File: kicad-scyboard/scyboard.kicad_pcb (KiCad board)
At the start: 2 copper layers, 144 x 96.5 mm, 76 parts

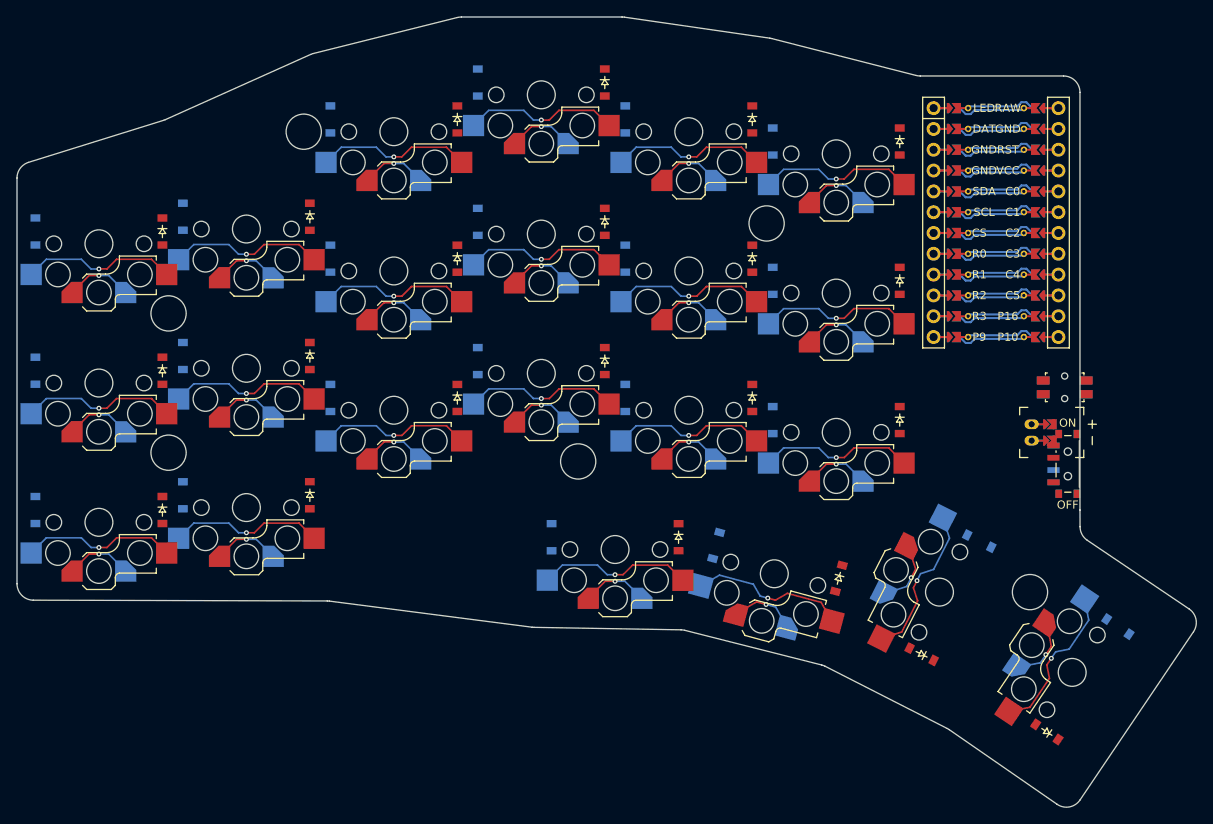
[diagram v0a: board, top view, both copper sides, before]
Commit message: Compile
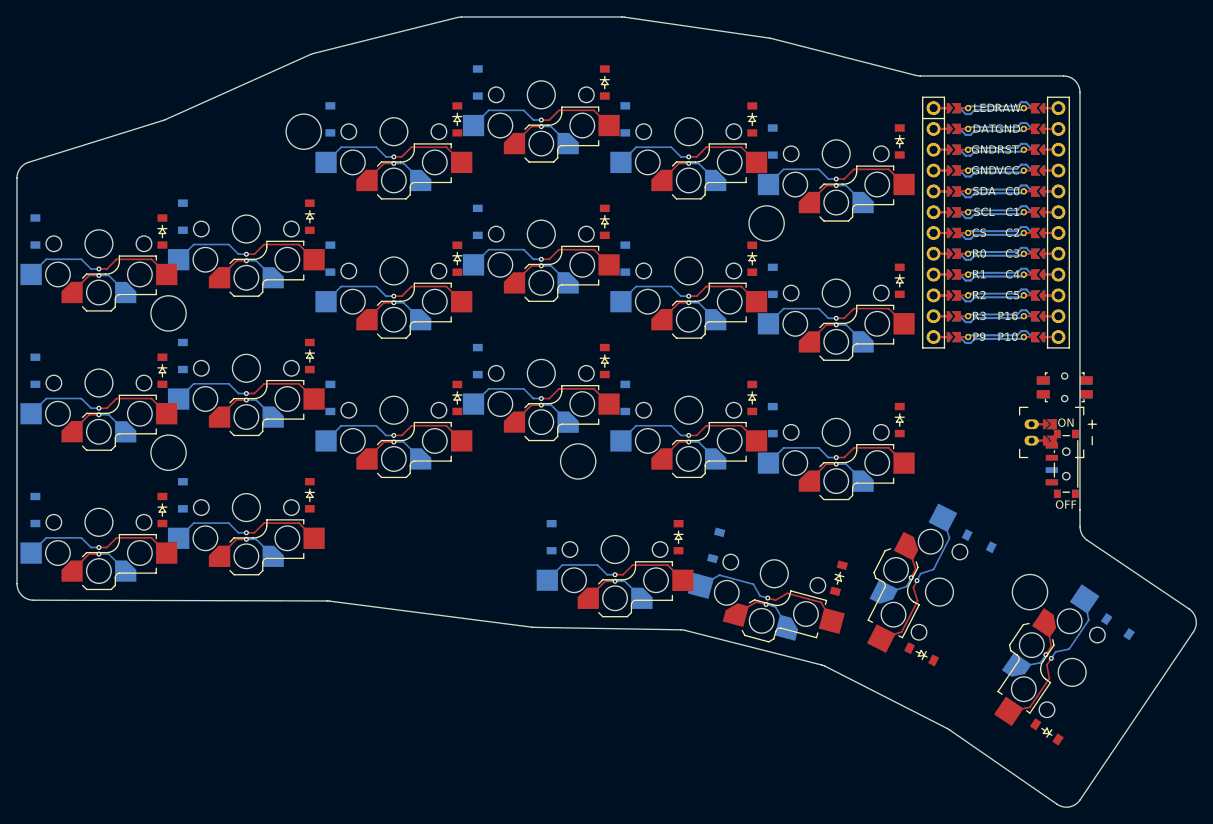
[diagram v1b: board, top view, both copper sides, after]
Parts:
- moved PWR1 0.19 mm to (168.1, 92.9)
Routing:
- net (no net): track 0.00 -> 337.7 mm
- net GND: track 29.5 -> 0.00 mm
- net P9: track 9.84 -> 0.00 mm
- net DAT: track 9.84 -> 0.00 mm
- net R2: track 9.84 -> 0.00 mm
- net LED: track 9.84 -> 0.00 mm
- net CS: track 9.84 -> 0.00 mm
- net SCL: track 9.84 -> 0.00 mm
- net SDA: track 9.84 -> 0.00 mm
- net R3: track 9.84 -> 0.00 mm
- net R1: track 9.84 -> 0.00 mm
- net R0: track 9.84 -> 0.00 mm
- net C4: track 42.9 -> 33.1 mm
- net C5: track 42.9 -> 33.1 mm
- net RAW: track 9.83 -> 0.00 mm
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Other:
- board size 144 x 96.5 mm -> 143.9 x 96.5 mm
